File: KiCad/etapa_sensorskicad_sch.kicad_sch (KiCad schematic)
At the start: 9 parts, among them J5 Conn_01x04_Pin, U23 FXTH87, U6 FDC2214

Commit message: Correccions dels sheets i títols fetes
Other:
- title: (none) -> Etapa de Sensors del projecte
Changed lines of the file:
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@@
 	(generator_version "9.0")
 	(paper "A4")
+	(title_block
+		(title "Etapa de Sensors del projecte")
+	)
 	(text "FXTH87 \n(Pressió)"
 		(exclude_from_sim no)

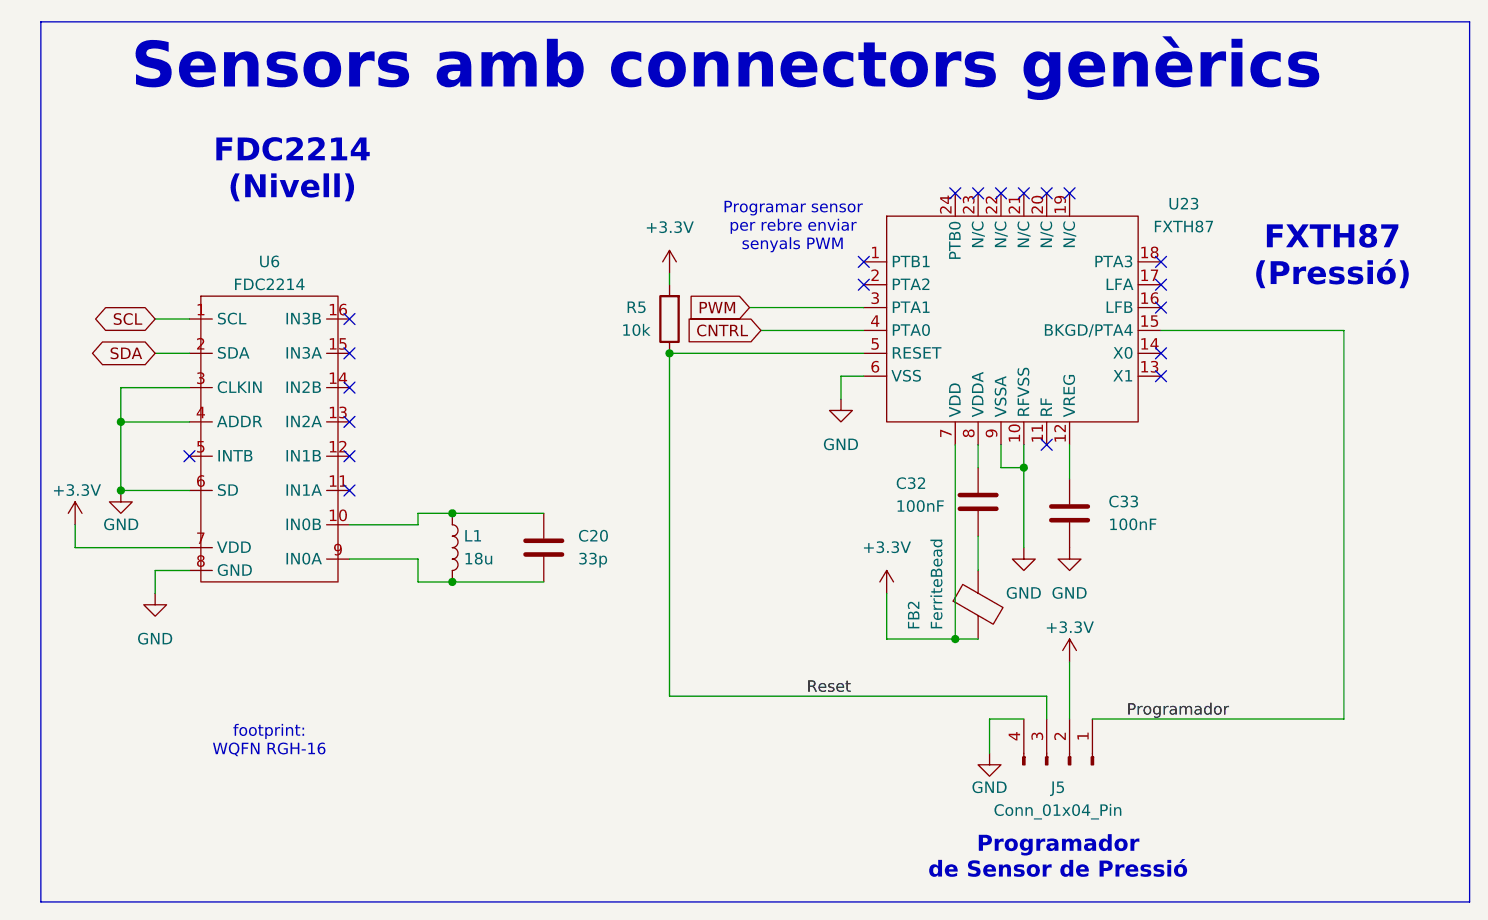
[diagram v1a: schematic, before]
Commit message: ALFRED DEGANOS SECOOOOS PLS DADDY ALFRED TE CAMELAMOS
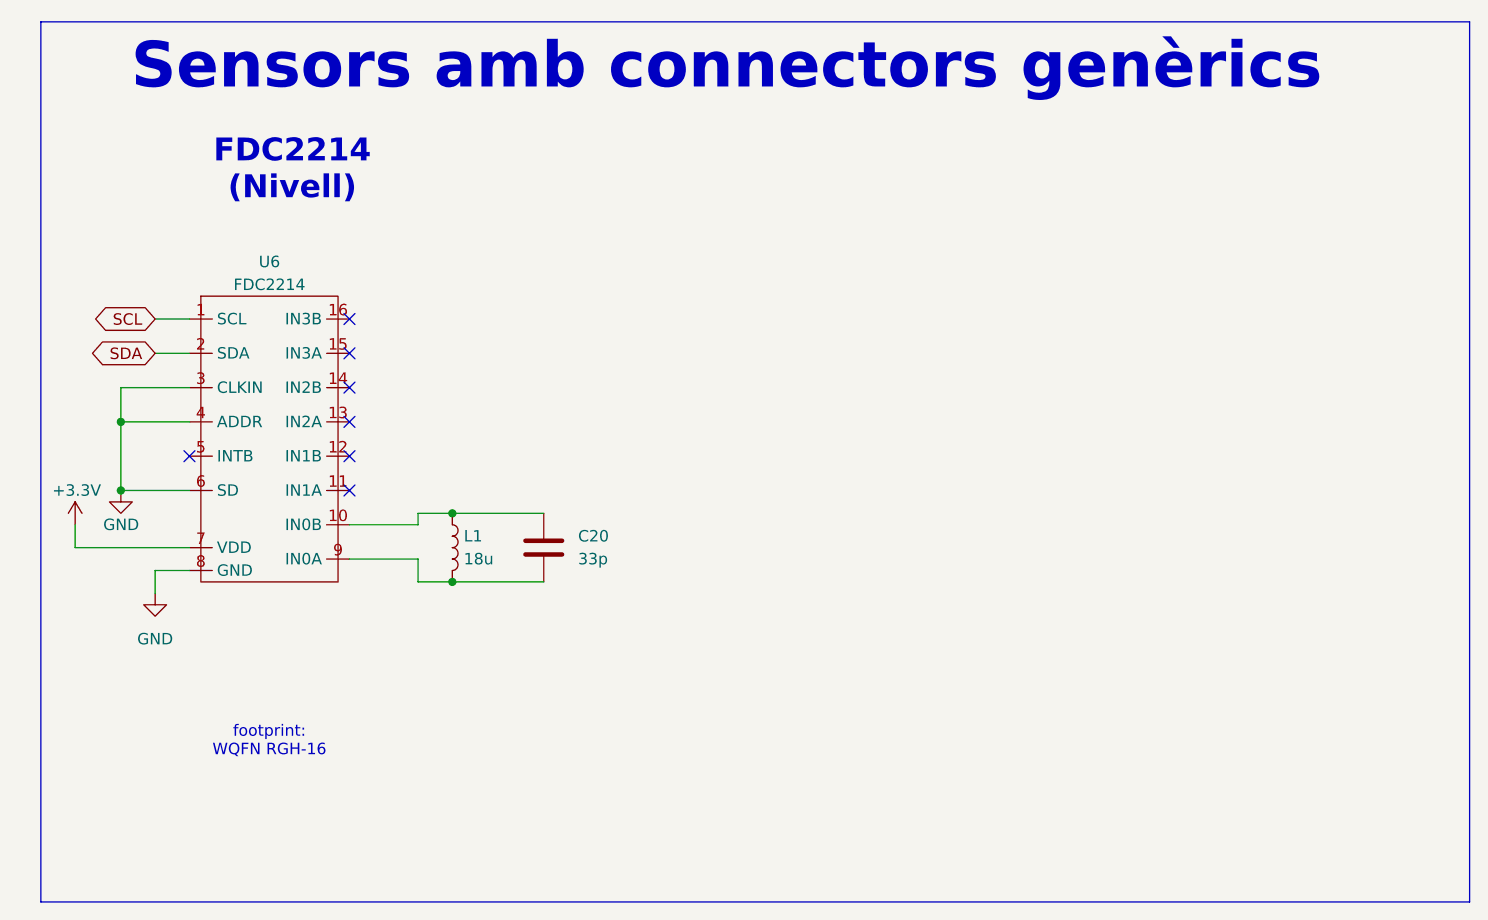
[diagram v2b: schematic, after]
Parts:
- removed C32, C33: 100nF, Capacitor_SMD:C_0805_2012Metric, symbol Device:C
- removed FB2: FerriteBead, Inductor_SMD:L_1812_4532Metric, symbol Device:FerriteBead
- removed J5: Conn_01x04_Pin, Connector_PinHeader_2.54mm:PinHeader_1x04_P2.54mm_Vertical, symbol Connector:Conn_01x04_Pin
- removed R5: 10k, Resistor_SMD:R_0805_2012Metric, symbol Device:R
- removed U23: FXTH87, Package_DFN_QFN:UDC-QFN-20-4EP_3x4mm_P0.5mm_EP0.41x0.25mm, symbol FXTH87:FXTH87
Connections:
- no-connect marks 21 -> 7
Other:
- note removed: "FXTH87 (Pressió)"
- note removed: "Programador de Sensor de Pressió"
- note removed: "Programar sensor per rebre enviar senyals PWM"
